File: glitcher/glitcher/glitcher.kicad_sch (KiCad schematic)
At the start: 4 parts, among them J1 Barrel_Jack, U1 SC0915, U2 CMOD_A7

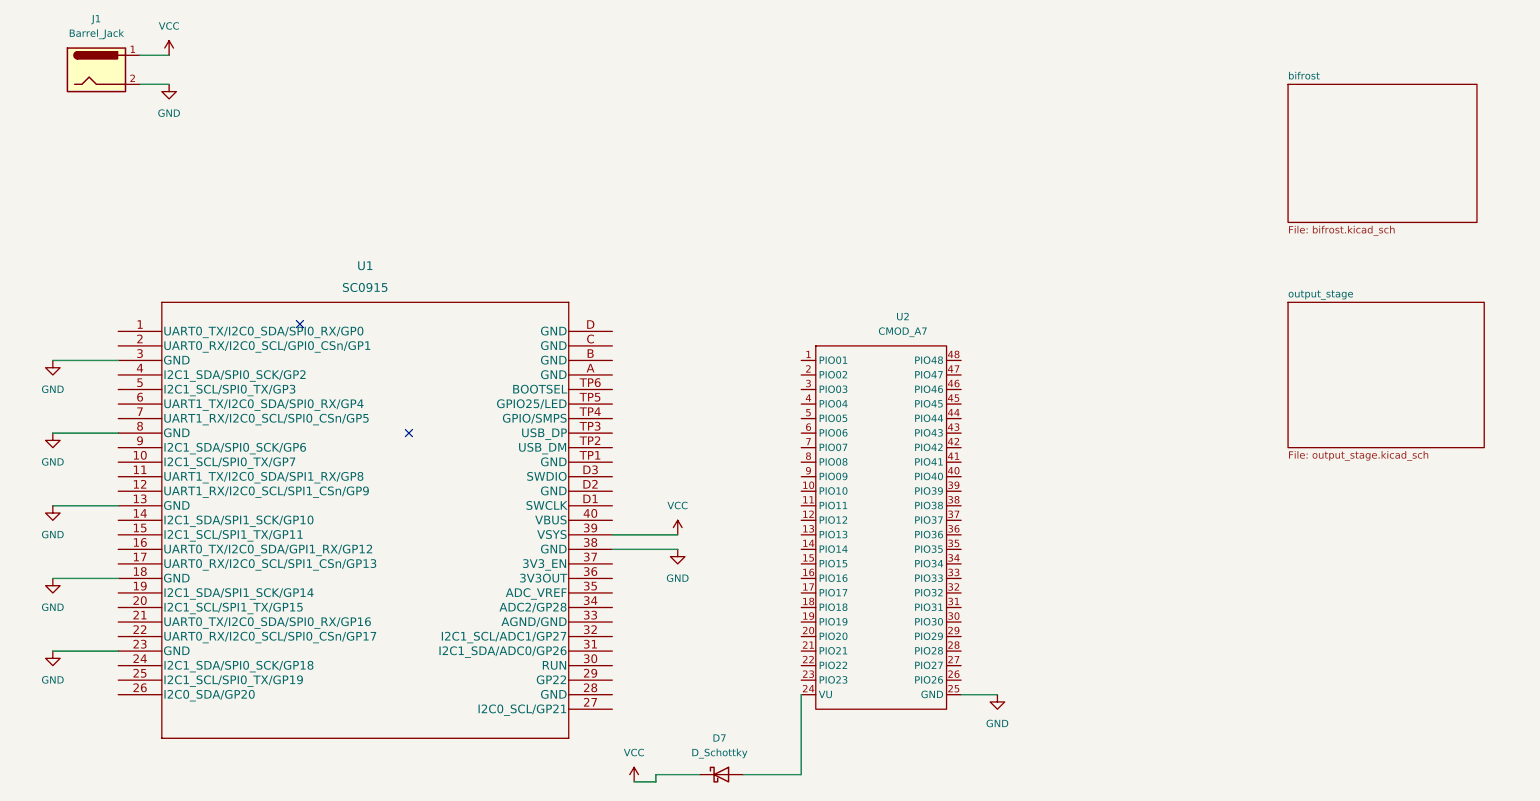
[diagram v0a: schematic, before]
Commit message: lolsave
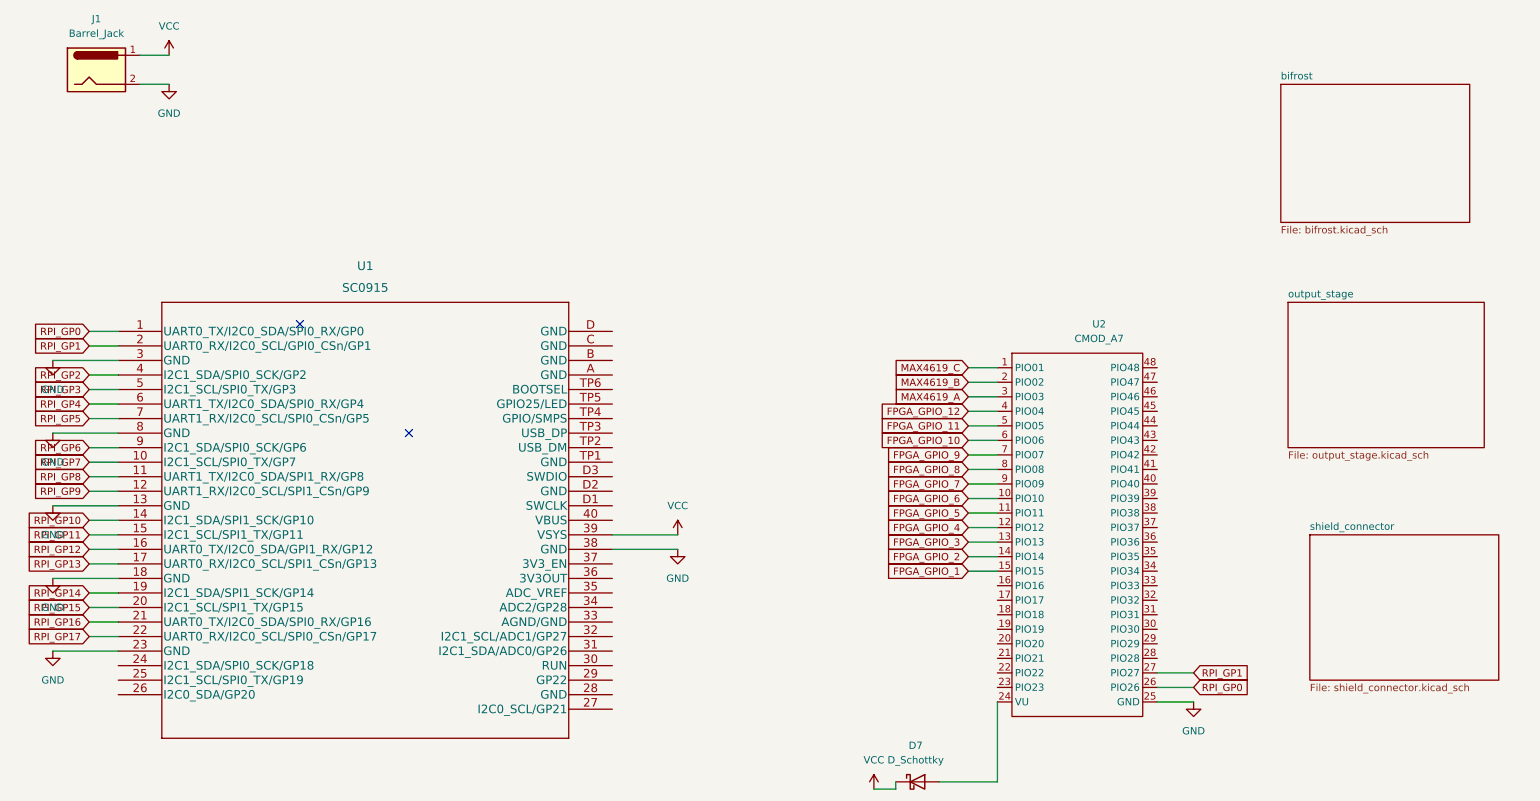
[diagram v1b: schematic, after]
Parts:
- D7: footprint (none) -> Diode_SMD:D_SOD-123F
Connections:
- net RPI_GP0: now reaches U1.1 (UART0_TX/I2C0_SDA/SPI0_RX/GP0)
- net RPI_GP0: now also U2.26 (PIO26)
- net RPI_GP7: now reaches U1.10 (I2C1_SCL/SPI0_TX/GP7)
- net RPI_GP8: now reaches U1.11 (UART1_TX/I2C0_SDA/SPI1_RX/GP8)
- net RPI_GP9: now reaches U1.12 (UART1_RX/I2C0_SCL/SPI1_CSn/GP9)
- net RPI_GP10: now reaches U1.14 (I2C1_SDA/SPI1_SCK/GP10)
- net RPI_GP11: now reaches U1.15 (I2C1_SCL/SPI1_TX/GP11)
- net RPI_GP12: now reaches U1.16 (UART0_TX/I2C0_SDA/GPI1_RX/GP12)
- net RPI_GP13: now reaches U1.17 (UART0_RX/I2C0_SCL/SPI1_CSn/GP13)
- net RPI_GP14: now reaches U1.19 (I2C1_SDA/SPI1_SCK/GP14)
- net RPI_GP1: now reaches U1.2 (UART0_RX/I2C0_SCL/GPI0_CSn/GP1)
- net RPI_GP1: now also U2.27 (PIO27)
- net RPI_GP15: now reaches U1.20 (I2C1_SCL/SPI1_TX/GP15)
- net RPI_GP16: now reaches U1.21 (UART0_TX/I2C0_SDA/SPI0_RX/GP16)
- net RPI_GP17: now reaches U1.22 (UART0_RX/I2C0_SCL/SPI0_CSn/GP17)
- net RPI_GP2: now reaches U1.4 (I2C1_SDA/SPI0_SCK/GP2)
- net RPI_GP3: now reaches U1.5 (I2C1_SCL/SPI0_TX/GP3)
- net RPI_GP4: now reaches U1.6 (UART1_TX/I2C0_SDA/SPI0_RX/GP4)
- net RPI_GP5: now reaches U1.7 (UART1_RX/I2C0_SCL/SPI0_CSn/GP5)
- net RPI_GP6: now reaches U1.9 (I2C1_SDA/SPI0_SCK/GP6)
- net MAX4619_C: now reaches U2.1 (PIO01)
- net FPGA_GPIO_6: now reaches U2.10 (PIO10)
- net FPGA_GPIO_5: now reaches U2.11 (PIO11)
- net FPGA_GPIO_4: now reaches U2.12 (PIO12)
- net FPGA_GPIO_3: now reaches U2.13 (PIO13)
- net FPGA_GPIO_2: now reaches U2.14 (PIO14)
- net FPGA_GPIO_1: now reaches U2.15 (PIO15)
- net MAX4619_B: now reaches U2.2 (PIO02)
- net MAX4619_A: now reaches U2.3 (PIO03)
- net FPGA_GPIO_12: now reaches U2.4 (PIO04)
- net FPGA_GPIO_11: now reaches U2.5 (PIO05)
- net FPGA_GPIO_10: now reaches U2.6 (PIO06)
- net FPGA_GPIO_9: now reaches U2.7 (PIO07)
- net FPGA_GPIO_8: now reaches U2.8 (PIO08)
- net FPGA_GPIO_7: now reaches U2.9 (PIO09)
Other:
- added sheet shield_connector (shield_connector.kicad_sch)
- moved on the sheet: D7, U2
